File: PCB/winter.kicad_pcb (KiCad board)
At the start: 2 copper layers, 352.1 x 101.2 mm, 152 parts, among them J1 Conn_01x04, SW1 SW_Push, SW10 SW_Push, SW11 SW_Push, SW12 SW_Push, SW13 SW_Push, SW14 SW_Push, SW15 SW_Push, SW16 SW_Push, SW17 SW_Push, SW18 SW_Push, SW19 SW_Push, SW2 SW_Push, SW20 SW_Push, SW21 SW_Push, SW22 SW_Push, SW23 SW_Push, SW24 SW_Push, SW25 SW_Push, SW26 SW_Push, SW27 SW_Push, SW28 SW_Push, SW29 SW_Push, SW3 SW_Push, SW30 SW_Push, SW31 SW_Push, SW32 SW_Push, SW33 SW_Push, SW34 SW_Push, SW35 SW_Push, SW36 SW_Push, SW37 SW_Push, SW38 SW_Push, SW39 SW_Push, SW4 SW_Push, SW40 SW_Push, SW41 SW_Push, SW42 SW_Push, SW43 SW_Push, SW44 SW_Push, SW45 SW_Push, SW46 SW_Push, SW47 SW_Push, SW48 SW_Push, SW49 SW_Push, SW5 SW_Push, SW50 SW_Push, SW51 SW_Push, SW52 SW_Push, SW53 SW_Push, SW54 SW_Push, SW55 SW_Push, SW56 SW_Push, SW57 SW_Push, SW58 SW_Push, SW59 SW_Push, SW6 SW_Push, SW60 SW_Push, SW61 SW_Push, SW62 SW_Push, SW63 SW_Push, SW64 SW_Push, SW65 SW_Push, SW66 RotaryEncoder_Switch, SW7 SW_Push, SW8 SW_Push, SW9 SW_Push

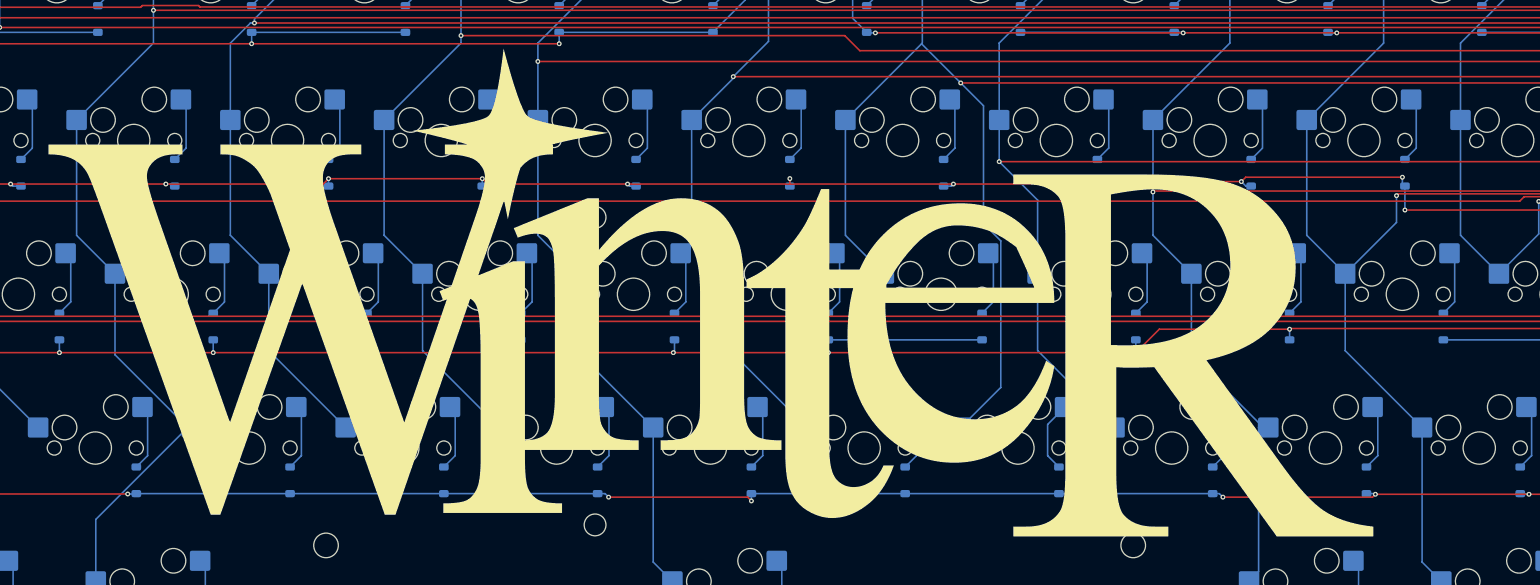
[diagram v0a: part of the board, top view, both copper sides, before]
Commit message: new branding and silkscreen
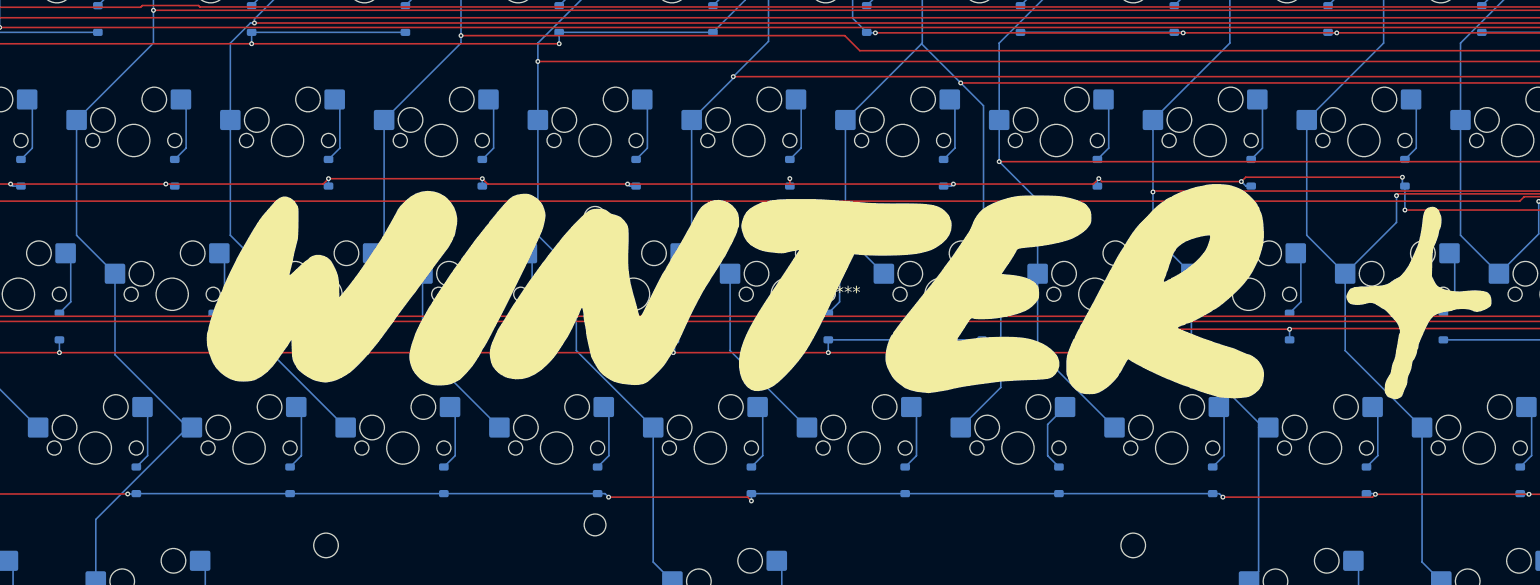
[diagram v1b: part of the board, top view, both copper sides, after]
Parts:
- added G***: LOGO, LOGO, F.Cu at (135.3, 37.9)
